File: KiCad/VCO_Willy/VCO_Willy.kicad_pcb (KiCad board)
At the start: 2 copper layers, 100 x 100 mm, 50 parts, among them J1 Conn_02x07_Odd_Even, J2 Conn_02x07_Odd_Even, J3 Conn_01x03_Male, J4 Conn_01x03_Male, J5 Conn_01x03_Male, U1 TL074, U2 TL074, U3 TL074

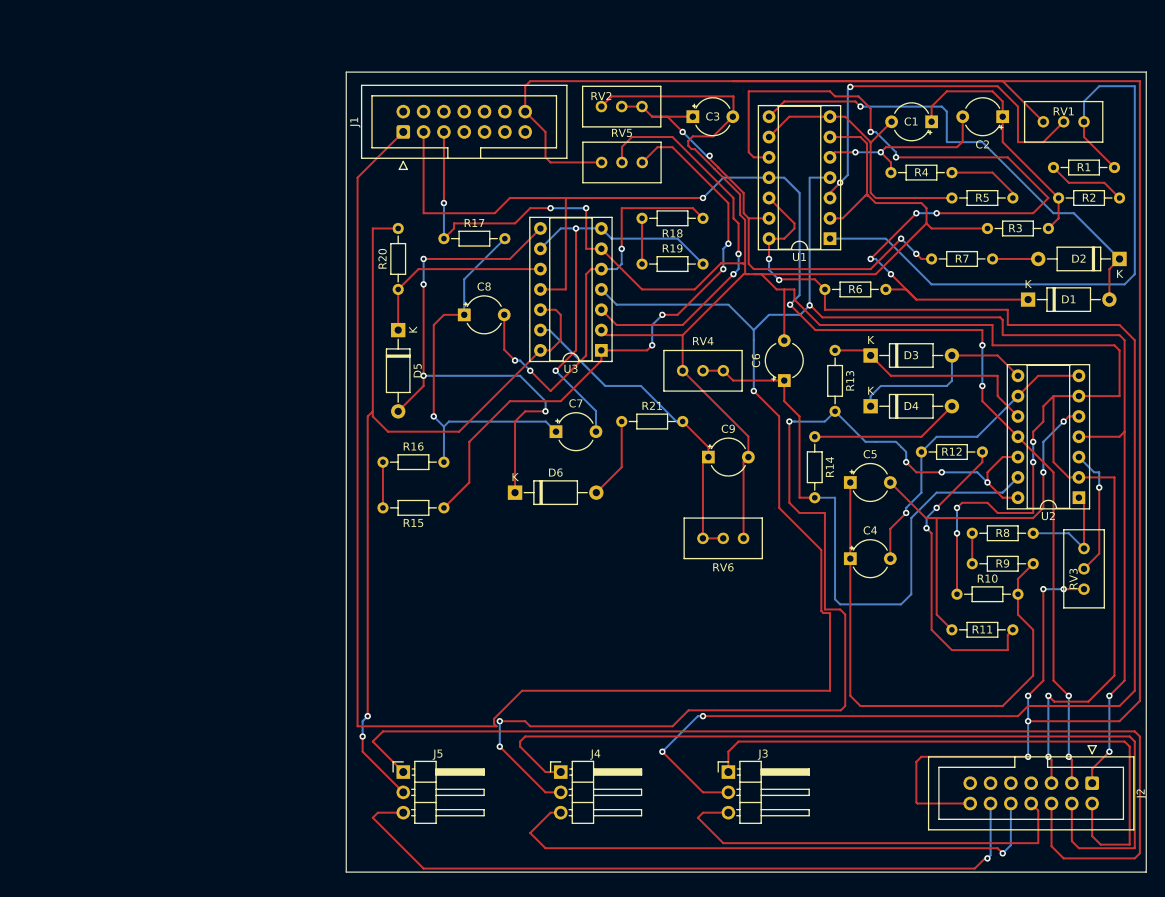
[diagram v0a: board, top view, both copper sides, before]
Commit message: upload new design
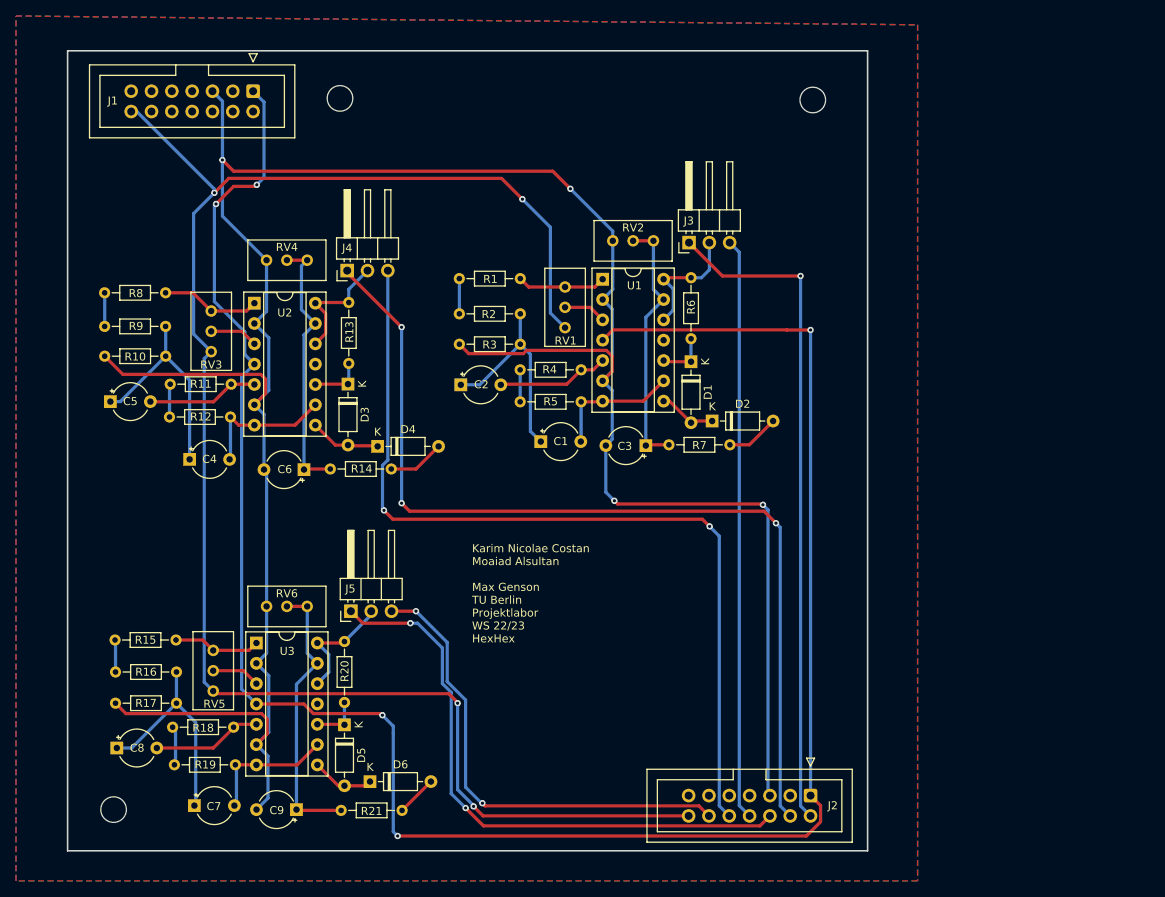
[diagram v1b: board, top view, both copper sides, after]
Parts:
- added REF**: MountingHole_3.2mm_M3, MountingHole:MountingHole_3.2mm_M3, F.Cu at (135.6, 57.4)
- added REF**: MountingHole_3.2mm_M3, MountingHole:MountingHole_3.2mm_M3, F.Cu at (194.7, 57.6)
- added REF**: MountingHole_3.2mm_M3, MountingHole:MountingHole_3.2mm_M3, F.Cu at (107.3, 146.3)
- D1, D2, D3, D4, D5, D6: footprint Diode_THT:D_A-405_P10.16mm_Horizontal -> Diode_THT:D_DO-35_SOD27_P7.62mm_Horizontal
- moved RV3 113.1 mm to (119.5, 84.0)
- moved R8 112.5 mm to (113.8, 81.7)
- moved R9 112.4 mm to (106.2, 85.9)
- moved R10 110.6 mm to (106.2, 89.6)
- moved U2 105.9 mm to (124.9, 83.0), turned to 0 degrees
- moved R12 101.7 mm to (114.3, 97.2), turned to 0 degrees
- moved R11 95.2 mm to (122.0, 93.1), turned to 180 degrees
- moved C5 93.0 mm to (106.9, 95.3)
- moved R18 86.5 mm to (122.3, 136.0)
- moved R19 85.6 mm to (114.9, 140.7)
- moved R2 83.8 mm to (150.5, 84.3), turned to 0 degrees
- moved C4 83.5 mm to (116.8, 102.5)
- moved RV5 81.2 mm to (119.8, 126.4), turned to 90 degrees
- moved C2 75.6 mm to (150.7, 93.2), turned to 0 degrees
- moved R1 75.6 mm to (158.1, 79.9)
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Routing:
- net Net-(J1-Pad3): track 175.5 -> 0.00 mm, vias 6 -> 0
- net Net-(J3-Pad2): track 181.2 -> 15.7 mm, vias 4 -> 0
- net Net-(J4-Pad2): track 139.3 -> 15.3 mm, vias 6 -> 0
- net Net-(D1-Pad1): track 107.0 -> 6.37 mm, vias 6 -> 0
- net Net-(J5-Pad2): track 111.9 -> 14.9 mm, vias 2 -> 0
- net Net-(J1-Pad1): track 341.3 -> 259.1 mm, vias 4 -> 5
- net Net-(C3-Pad2): track 390.2 -> 315.1 mm, vias 9 -> 4
- net Net-(R1-Pad1): track 81.5 -> 11.1 mm
- net Net-(J1-Pad14): track 280.6 -> 210.9 mm, vias 5 -> 4
- net Net-(R15-Pad1): track 75.5 -> 11.0 mm, vias 4 -> 0
- net Net-(J2-Pad6): track 133.9 -> 74.0 mm, vias 0 -> 2
- net Net-(D5-Pad2): track 67.6 -> 7.87 mm, vias 4 -> 0
- net Net-(D1-Pad2): track 60.6 -> 7.27 mm, vias 1 -> 0
- net Net-(C6-Pad1): track 78.5 -> 33.6 mm
- net Net-(RV5-Pad2): track 49.5 -> 6.07 mm, vias 2 -> 0
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- added copper zone on B.Cu, net Net-(J1-Pad3)
- added copper zone on F.Cu, net Net-(J1-Pad3)
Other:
- board text added: "Karim Nicolae Costan Moaiad Alsultan Max Genson TU Berlin Projektlabor WS 22/23 HexHex"
